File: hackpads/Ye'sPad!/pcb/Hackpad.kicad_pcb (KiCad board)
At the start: 2 copper layers, 99.5 x 77 mm, 31 parts, among them SW1 SW_Push, SW10 SW_Push, SW11 SW_Push, SW13 SW_Push, SW14 SW_Push, SW15 SW_Push, SW2 SW_Push, SW3 SW_Push, SW4 SW_Push, SW5 SW_Push, SW6 SW_Push, SW7 SW_Push, SW9 SW_Push, U1 MOUDLE-SEEEDUINO-XIAO

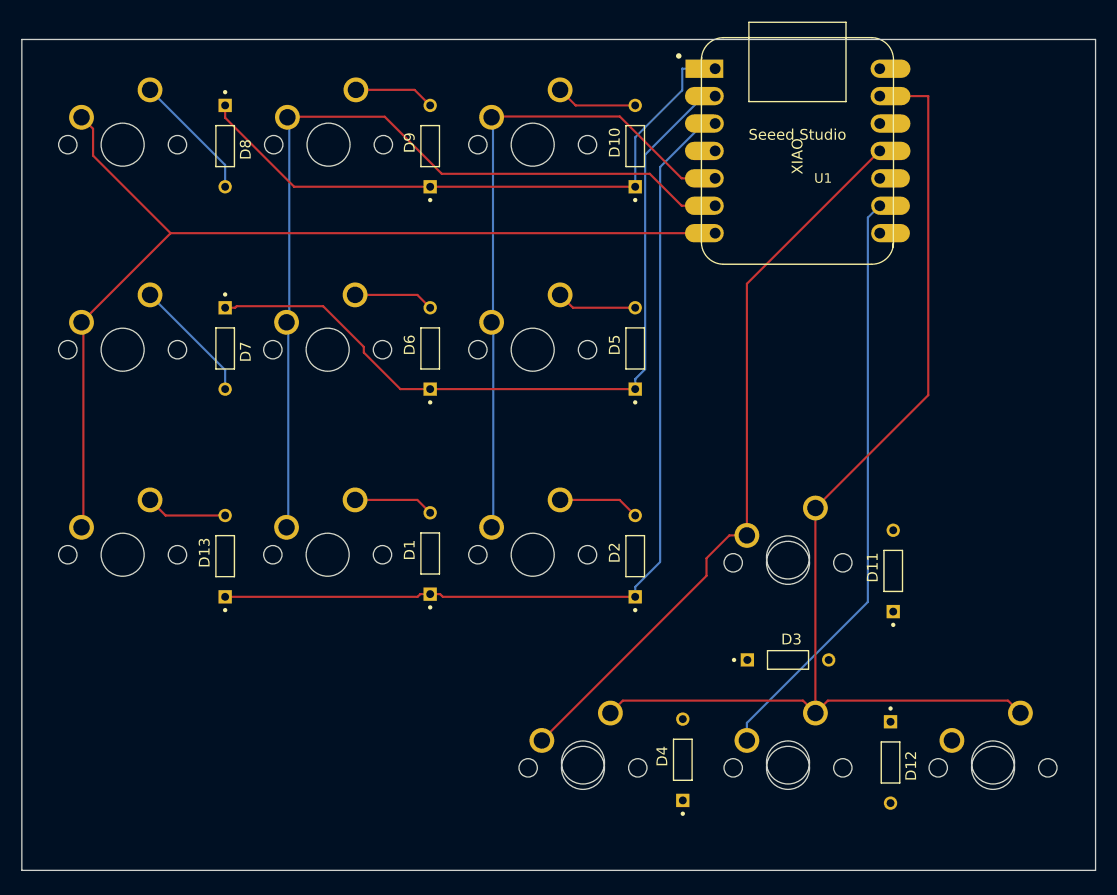
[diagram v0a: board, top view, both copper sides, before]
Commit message: Add files via upload
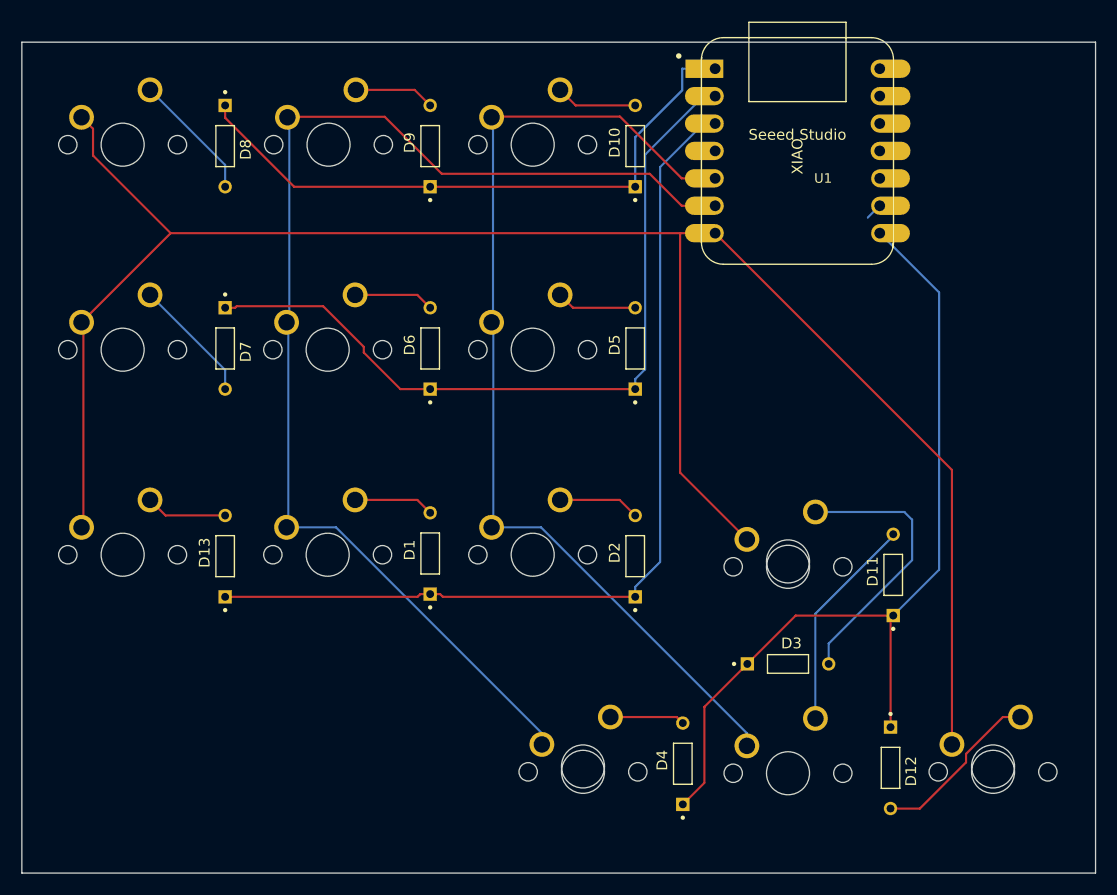
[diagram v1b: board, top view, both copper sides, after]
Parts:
- removed the ? at (134.2, 161.2)
- moved D12 0.50 mm to (143.8, 161.8)
- moved SW3 0.50 mm to (134.2, 162.2)
- moved ? 0.37 mm to (115.2, 161.6)
- moved ? 0.37 mm to (134.2, 142.6)
- moved ? 0.37 mm to (153.2, 161.6)
- moved D11 0.37 mm to (144.0, 143.9)
- moved D3 0.37 mm to (134.2, 152.1)
- moved D4 0.37 mm to (124.5, 161.4)
- moved SW1 0.37 mm to (134.2, 143.1)
- moved SW2 0.37 mm to (115.2, 162.1)
- moved SW4 0.37 mm to (153.2, 162.1)
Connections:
- D11 pad 1: (no net) -> row 3
- D11 pad 2: (no net) -> Net-(D11-A)
- D12 pad 1: (no net) -> row 3
- D12 pad 2: (no net) -> Net-(D12-A)
- D3 pad 1: (no net) -> row 3
- D3 pad 2: (no net) -> Net-(D3-A)
- D4 pad 1: (no net) -> row 3
- D4 pad 2: (no net) -> Net-(D4-A)
- SW1 pad 1: Net-(U1-PA6_A10_D10_MOSI) -> column 3
- SW1 pad 2: GND -> Net-(D3-A)
- SW2 pad 1: Net-(U1-PA6_A10_D10_MOSI) -> column 2
- SW2 pad 2: GND -> Net-(D4-A)
- SW3 pad 1: Net-(U1-PA7_A8_D8_SCK) -> column 1
- SW3 pad 2: GND -> Net-(D11-A)
- SW4 pad 1: Net-(U1-PB09_A7_D7_RX) -> column 4
- SW4 pad 2: GND -> Net-(D12-A)
- U1 pad 10: Net-(U1-PA5_A9_D9_MISO) -> unconnected-(U1-PA5_A9_D9_MISO-Pad10)
- U1 pad 11: Net-(U1-PA6_A10_D10_MOSI) -> unconnected-(U1-PA6_A10_D10_MOSI-Pad11)
- U1 pad 13: GND -> unconnected-(U1-GND-Pad13)
- U1 pad 7: column 3 -> column 4
- U1 pad 8: unconnected-(U1-PB09_A7_D7_RX-Pad8) -> row 3
- U1 pad 9: Net-(U1-PA7_A8_D8_SCK) -> unconnected-(U1-PA7_A8_D8_SCK-Pad9)
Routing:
- net GND: track 106.2 -> 0.00 mm
- net row 3: track 0.00 -> 80.8 mm
- net Net-(U1-PA6_A10_D10_MOSI): track 70.1 -> 0.00 mm
- net column 4: track 0.00 -> 56.1 mm
- net Net-(U1-PA7_A8_D8_SCK): track 55.3 -> 0.00 mm
- net column 1: track 61.4 -> 94.1 mm
- net column 2: track 81.4 -> 114.0 mm
- net column 3: track 95.5 -> 126.4 mm
- net Net-(D3-A): track 0.00 -> 25.8 mm
- net Net-(D11-A): track 0.00 -> 20.1 mm
- net Net-(D12-A): track 0.00 -> 16.0 mm
- net Net-(D4-A): track 0.00 -> 6.94 mm
- net unconnected-(U1-PA7_A8_D8_SCK-Pad9): track 0.00 -> 1.56 mm
